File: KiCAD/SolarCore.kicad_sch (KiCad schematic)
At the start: 26 parts, among them SW1 SW_SPST, U1 LMR33630ARNXR, U2 NUCLEO-L432KC

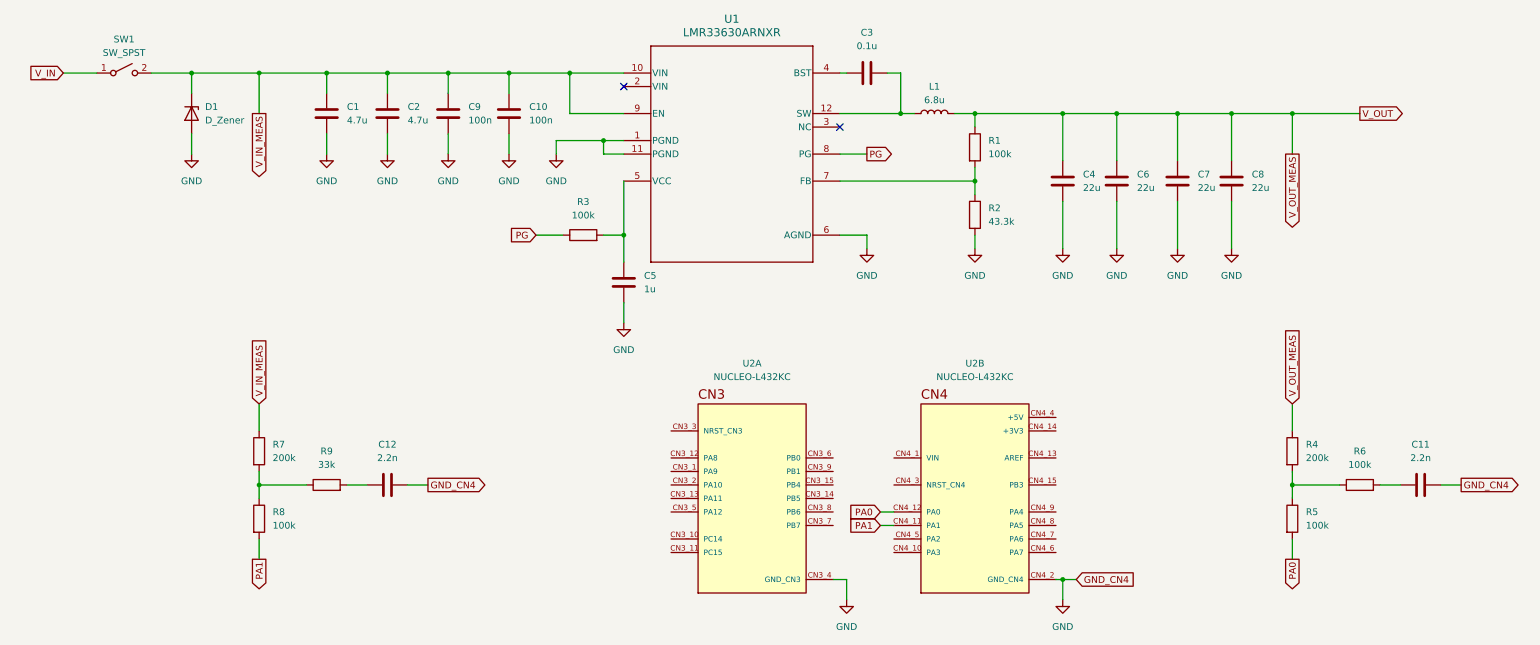
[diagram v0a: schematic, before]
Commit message: Final schematic V1
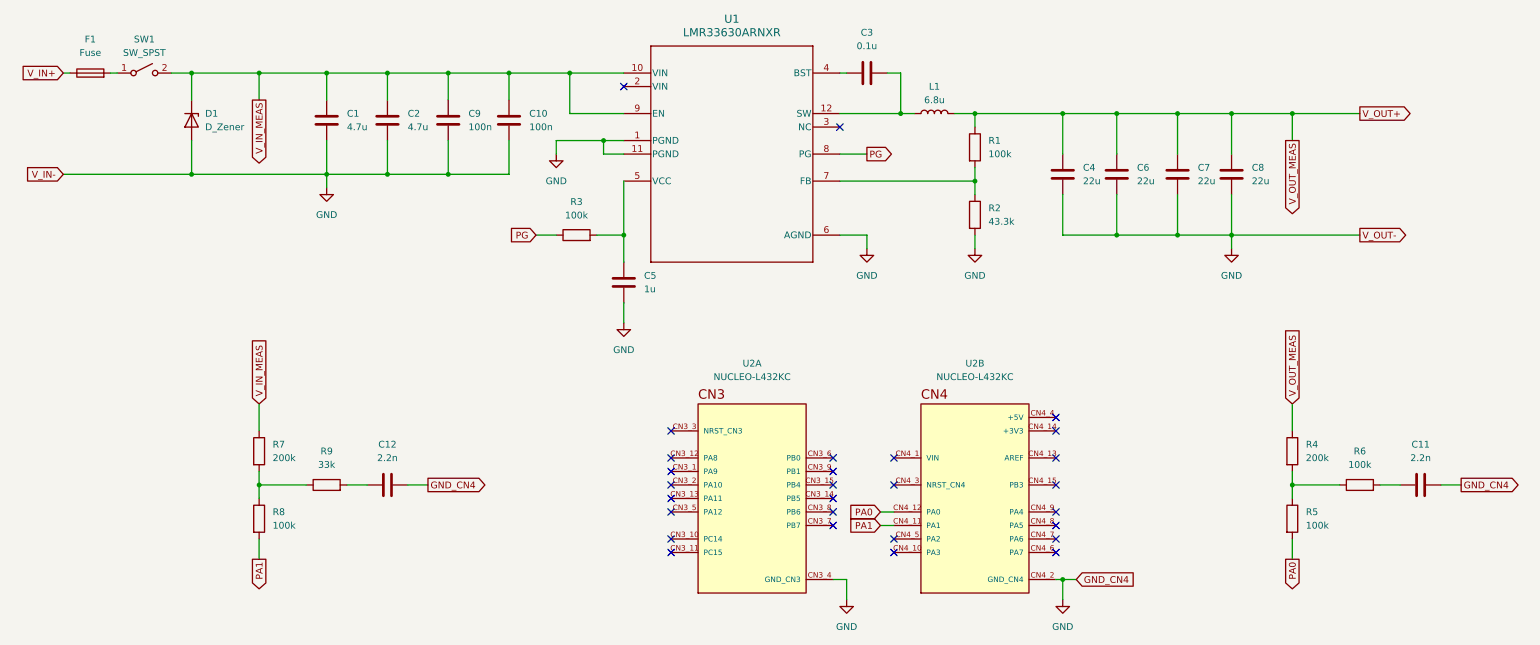
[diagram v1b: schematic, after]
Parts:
- added F1: Fuse, Fuse:Fuse_2512_6332Metric_Pad1.52x3.35mm_HandSolder, symbol Device:Fuse
- SW1: footprint (none) -> Connector_JST:JST_VH_B2P-VH_1x02_P3.96mm_Vertical
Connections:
- net V_IN: no longer names the net of SW1.1 (A)
- net V_IN: now also F1.2
- net V_OUT renamed V_OUT+
- new net V_IN+: F1.1
- no-connect marks 2 -> 28
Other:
- moved on the sheet: C1, C10, C2, C4, C6, C7, C8, C9, D1, R3, SW1
